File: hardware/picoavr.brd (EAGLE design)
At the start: 37.2 x 20.3 mm, 26 parts, among them IC1 MCP1703CB, Q2 12mhz, SW1 SPST_TACT-KMR2, U3 ATMEGA328P, X1 Micro USB

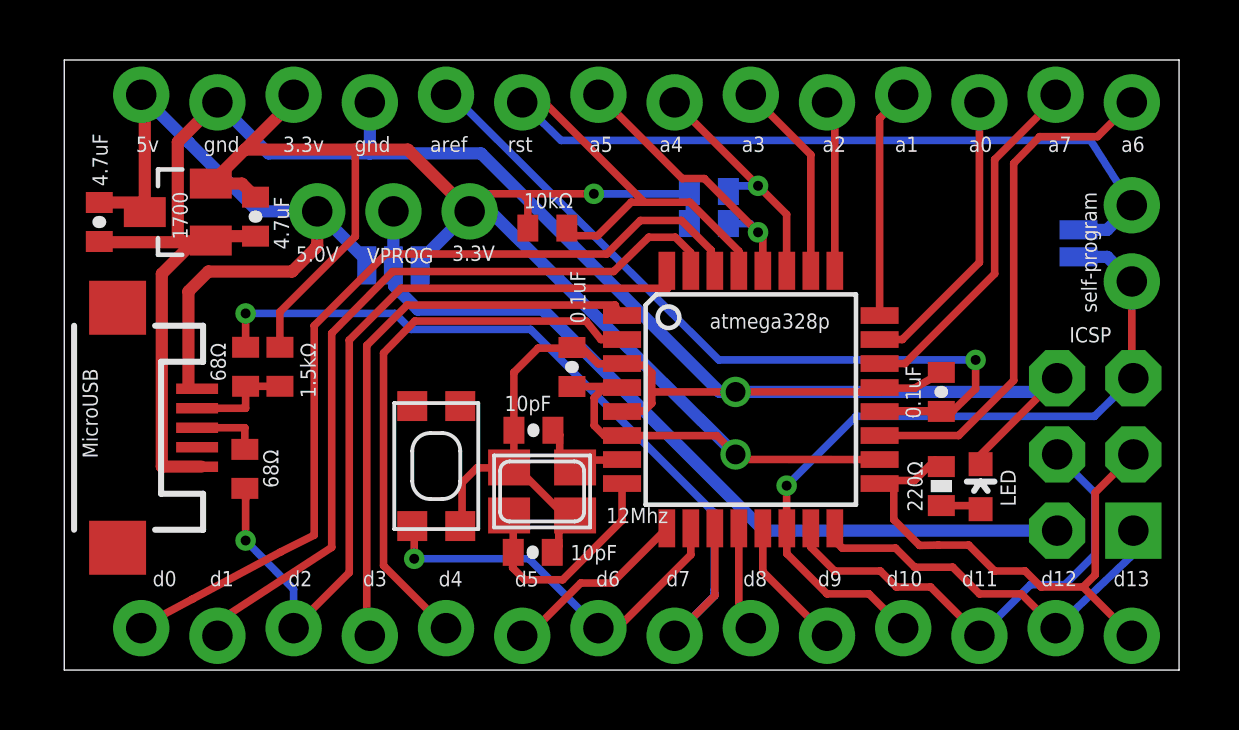
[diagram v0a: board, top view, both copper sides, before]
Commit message: new hardware revision
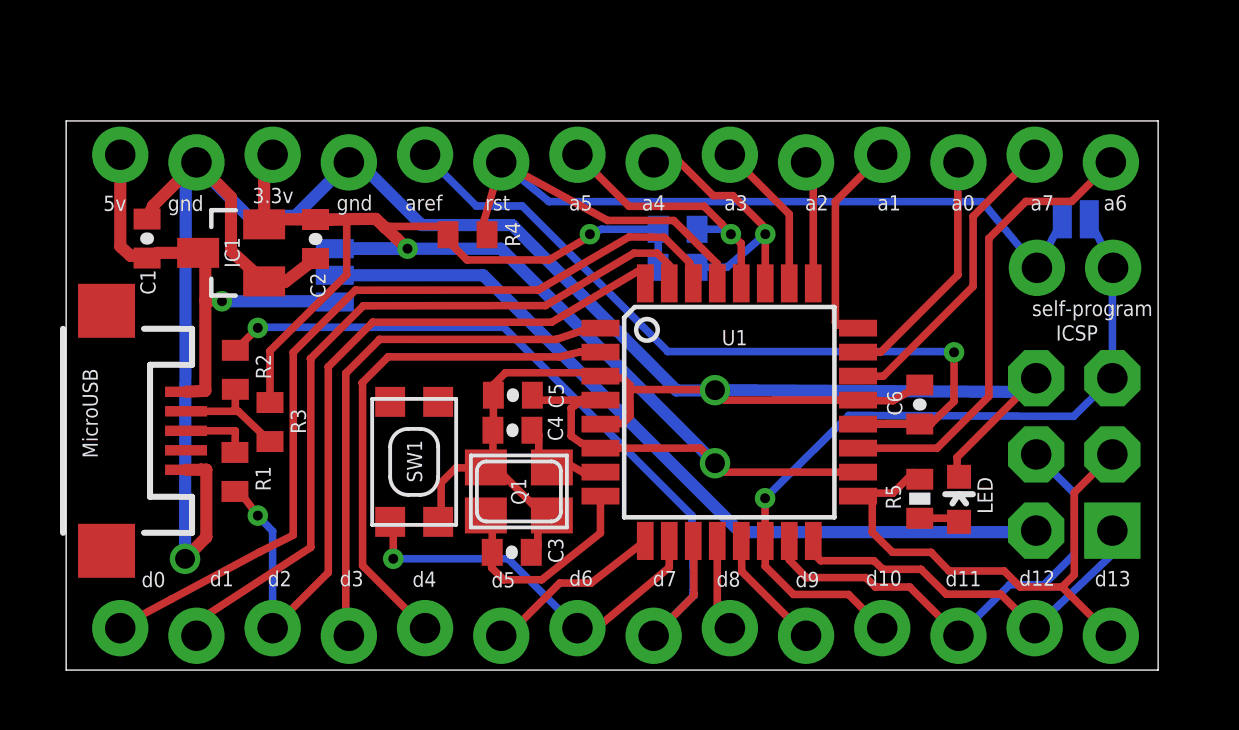
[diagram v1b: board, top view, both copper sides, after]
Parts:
- removed LED2: GREEN, SparkFun:LED-0603
- removed POWER: (no value), SparkFun-Connectors:1X03_NO_SILK
- removed R9: 220, SparkFun:0402-RES
- added LED: GREEN, SparkFun:LED-0603
- added R4: 10k, resistor:R0402
- R1, R2: value 4.7k -> 68; device SparkFun:0402-RES -> resistor:R0402
- R3: value 68 -> 1.5k
- R5: value 68 -> 220; device resistor:R0402 -> SparkFun:0402-RES
- R6: value 10k -> 4.7k; device resistor:R0402 -> SparkFun:0402-RES
- R7: value 1.5k -> 4.7k; device resistor:R0402 -> SparkFun:0402-RES
- moved R5 22.5 mm to (28.5, 5.71)
- moved R1 18.4 mm to (5.66, 6.60), flipped to the top, turned to 270 degrees
- moved R2 16.5 mm to (5.68, 10.0), flipped to the top, turned to 90 degrees
- moved R7 14.0 mm to (20.4, 14.7), flipped to the bottom, turned to 180 degrees
- moved R6 4.54 mm to (20.4, 13.4), flipped to the bottom, turned to 180 degrees
- moved SELF_PROGRAM 3.79 mm to (32.4, 13.4), turned to 0 degrees
- moved IC1 2.24 mm to (5.54, 13.9)
- moved C5 2.18 mm to (14.9, 9.16), turned to 180 degrees
- moved C2 2.14 mm to (8.35, 14.4)
- moved JP3 2.12 mm to (1.84, 17.1)
- moved R3 2.01 mm to (6.83, 8.27)
- moved SJ1 1.98 mm to (8.99, 13.2), turned to 90 degrees
- moved C1 1.69 mm to (2.74, 14.4), turned to 90 degrees
- moved C6 0.83 mm to (28.5, 8.85)
- moved U3 0.83 mm to (22.1, 8.60)
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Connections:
- net GND: now also LED.C; no longer LED2.C
- net N$11: now also LED.A, R5.2; no longer LED2.A, R9.2
- net N$2: now also R1.1; no longer R5.1
- net N$4: now also R2.1; no longer R7.1
- net RESET: now also R4.2; no longer R6.2
- net SCK: now also R5.1; no longer R9.1
- net SCL: now also R7.2; no longer R2.2
- net SDA: now also R6.2; no longer R1.2
- net USB_DMINUS: now also R2.2; no longer R3.2
- net USB_DPLUS: now also R1.2; no longer R5.2
- net USB_VBUS: no longer POWER.1
- net VCC: now also R3.2, R4.1, R7.1; no longer POWER.3, R1.1, R2.1, R7.2
- net VPROG: no longer POWER.2
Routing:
- net USB_VBUS: track 25.7 -> 15.9 mm, vias 0 -> 1
- net RESET: track 38.0 -> 33.1 mm
- net GND: track 88.8 -> 93.0 mm, vias 1 -> 2
- net USB_DPLUS: track 28.4 -> 26.6 mm
- net A6: track 17.3 -> 15.5 mm
- net A2: track 5.87 -> 4.13 mm
- net USB_DMINUS: track 28.5 -> 26.8 mm
- net A3: track 6.70 -> 5.11 mm
- net A0: track 9.73 -> 8.16 mm
- net A7: track 11.8 -> 10.3 mm
- net ISP_RESET: track 25.6 -> 26.9 mm
- net D4: track 18.7 -> 17.4 mm
- net D3: track 19.3 -> 18.1 mm
- net D0: track 29.3 -> 28.3 mm
- net VPROG: track 28.0 -> 26.9 mm
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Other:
- board size 37.2 x 20.3 mm -> 36.4 x 18.3 mm
- board text added: "C1"
- board text added: "C2"
- board text added: "C3"
- board text added: "C4"
- board text added: "C5"
- board text added: "C6"
- board text added: "IC1"
- board text added: "PicoAVR rev 1.3"
- board text added: "Q1"
- board text added: "R1"
- board text added: "R2"
- board text added: "R3"
- board text added: "R4"
- board text added: "R5"
- board text added: "SW1"
- board text added: "U1"
- board text removed: "0.1uF"
- board text removed: "1.5kΩ"
- board text removed: "10kΩ"
- board text removed: "10pF"
- board text removed: "12Mhz"
- board text removed: "1700"
- board text removed: "220Ω"
- board text removed: "3.3V"
- board text removed: "4.7kΩ (SCL)"
- board text removed: "4.7kΩ (SDA)"
- board text removed: "4.7uF"
- board text removed: "5.0V"
- board text removed: "68Ω"
- board text removed: "PicoAVR rev 1.2"
- board text removed: "VPROG"
- board text removed: "atmega328p"
